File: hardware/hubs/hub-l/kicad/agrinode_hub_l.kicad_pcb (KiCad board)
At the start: 2 copper layers, 130 x 96 mm, 105 parts, among them J1 DC 12V 5.5/2.1, J2 DC IN 7-24V, J3 SOLAR 6-24V, J4 USB 5V / PROG, J5 BAT NTC 10k, J6 PROG, J7 I2C, J8 LED STRIP WS2813, J9 RS-485, Q1 AO3401A, Q2 AO3401A, Q3 MMBT3904, Q4 MMBT3904, Q5 BSS138, Q6 MMBT3904, SW1 RESET, SW2 BOOT / PAIR, U1 LM2596S-5.0, U2 TP4056, U3 MIC29302WU, U4 ESP32-WROOM-32E-N8, U5 CH340C, U6 DS3231MZ, U7 MAX3485ESA, U8 Ra-02 SX1278 433MHz

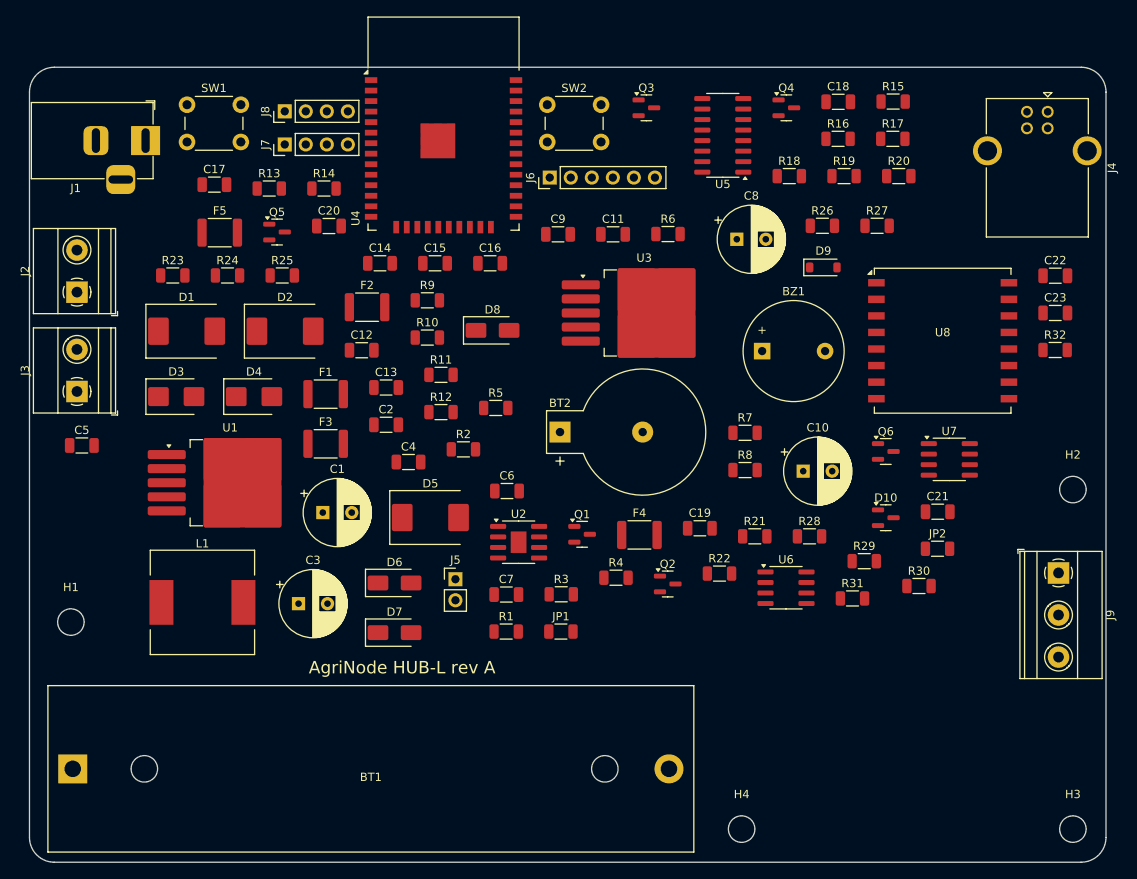
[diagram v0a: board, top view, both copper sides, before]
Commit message: hubs: routing progress snapshot (HUB-L 3 open)
Co-Authored-By: Claude Opus 5.5 <noreply@anthropic.com>
Claude-Session: https://claude.ai/code/session_014J7amXZ5Y6AZWEh5CjDNja
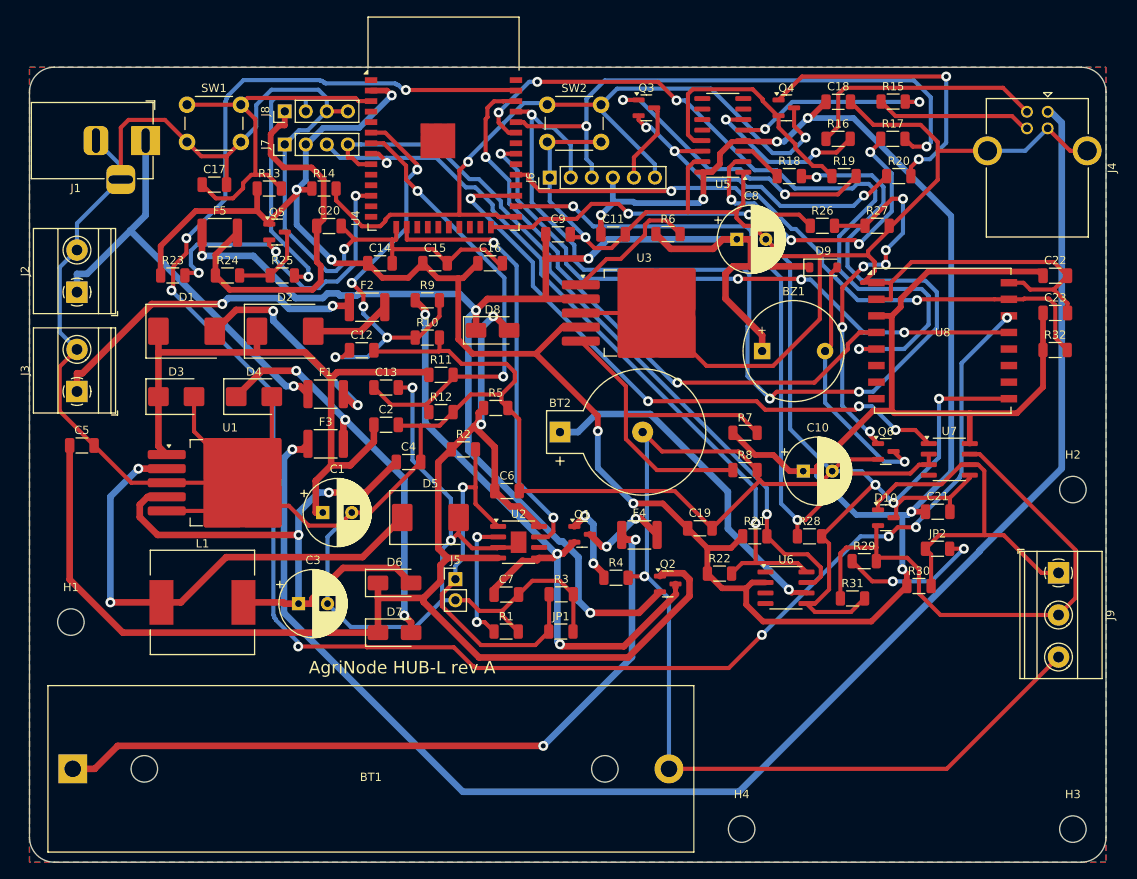
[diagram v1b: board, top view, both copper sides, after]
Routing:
- net GND: track 0.00 -> 884.8 mm, vias 0 -> 8
- net +3V3: track 0.00 -> 399.1 mm, vias 0 -> 11
- net SPI_MOSI: track 0.00 -> 223.6 mm, vias 0 -> 8
- net /Power - 12V, solar and USB inputs, 18650 charger, rails/VUSB_RAW: track 0.00 -> 185.4 mm, vias 0 -> 1
- net /Power - 12V, solar and USB inputs, 18650 charger, rails/V5: track 0.00 -> 177.7 mm, vias 0 -> 2
- net VSYS: track 0.00 -> 177.2 mm, vias 0 -> 4
- net /ESP32, programming, buttons, RTC, LED strip, buzzer/ESP_TXD0: track 0.00 -> 132.4 mm, vias 0 -> 4
- net /ESP32, programming, buttons, RTC, LED strip, buzzer/BOOT_BTN: track 0.00 -> 96.7 mm, vias 0 -> 2
- net LORA_DIO0: track 0.00 -> 95.4 mm, vias 0 -> 4
- net /ESP32, programming, buttons, RTC, LED strip, buzzer/I2C_SCL: track 0.00 -> 92.5 mm, vias 0 -> 2
- net /ESP32, programming, buttons, RTC, LED strip, buzzer/I2C_SDA: track 0.00 -> 91.0 mm, vias 0 -> 1
- net /Power - 12V, solar and USB inputs, 18650 charger, rails/BATT_CELL: track 0.00 -> 89.4 mm, vias 0 -> 2
- net RS485_DE: track 0.00 -> 88.7 mm, vias 0 -> 2
- net /Power - 12V, solar and USB inputs, 18650 charger, rails/VBAT: track 0.00 -> 79.6 mm, vias 0 -> 3
- net LORA_CS: track 0.00 -> 79.1 mm, vias 0 -> 2
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- added copper zone on B.Cu, net GND
- added copper zone on F.Cu, net GND
